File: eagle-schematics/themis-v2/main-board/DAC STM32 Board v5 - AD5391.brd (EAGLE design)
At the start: 161.3 x 134.6 mm, 229 parts, among them IC1 MCP23017SO, U1 ANALOG_DEVICES_AD5391BSTZ-3AN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

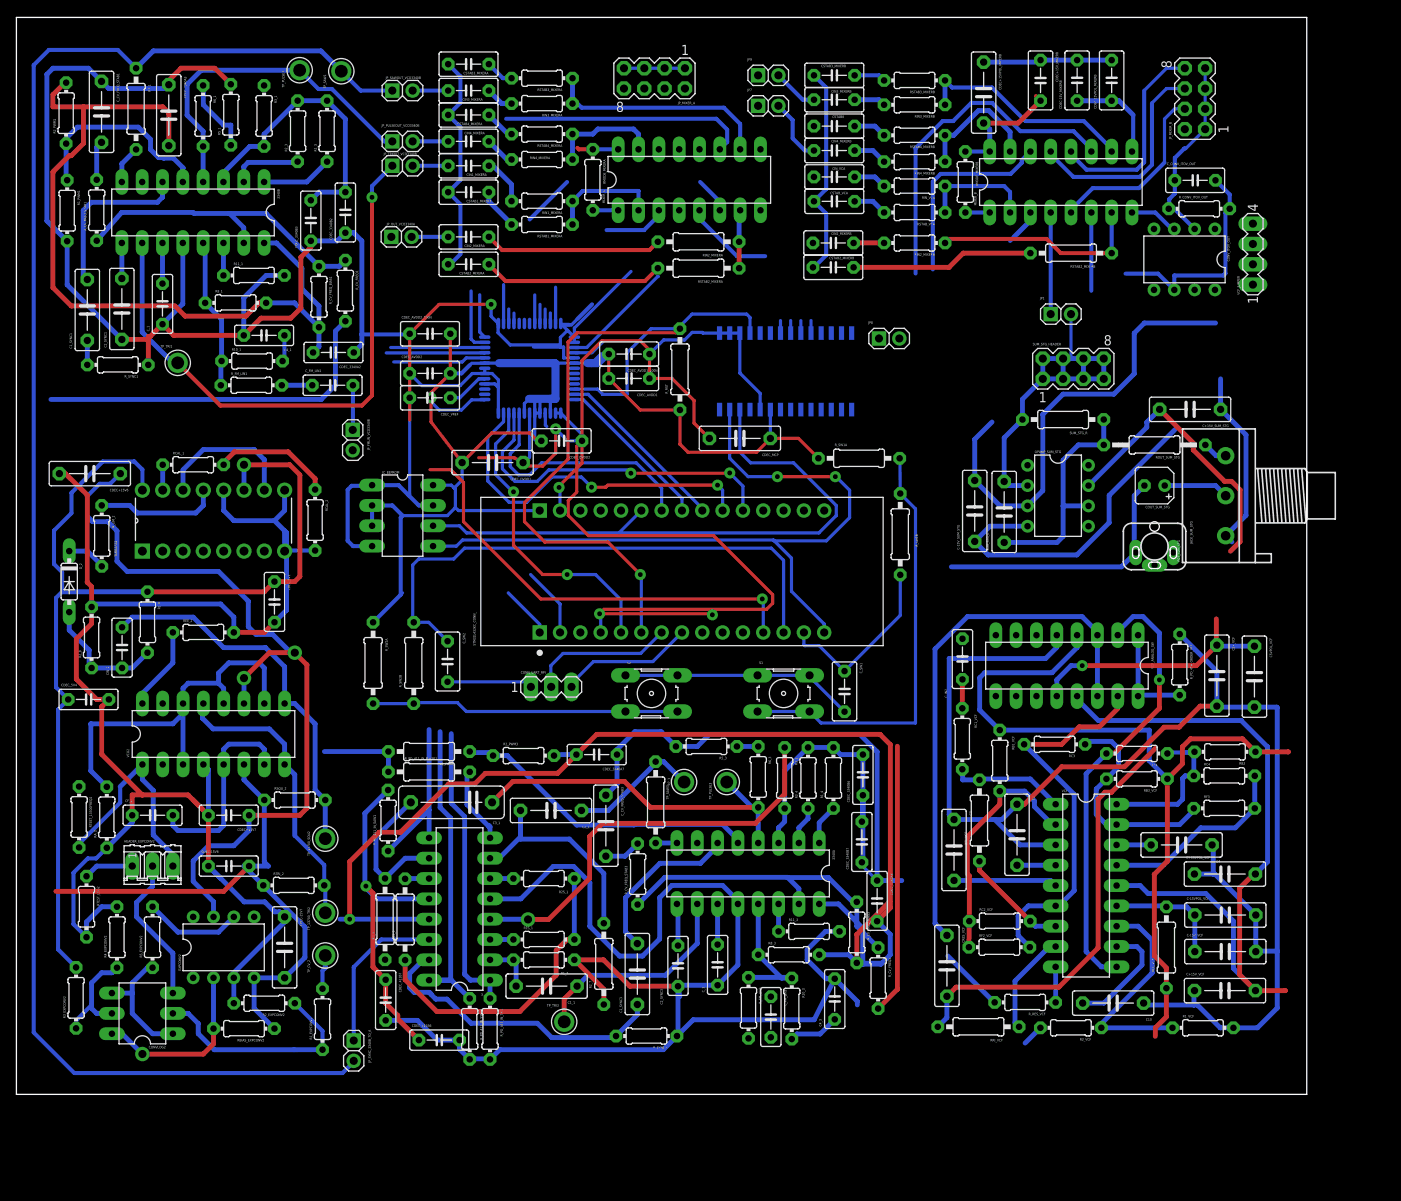
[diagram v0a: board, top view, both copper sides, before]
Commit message: bug fix
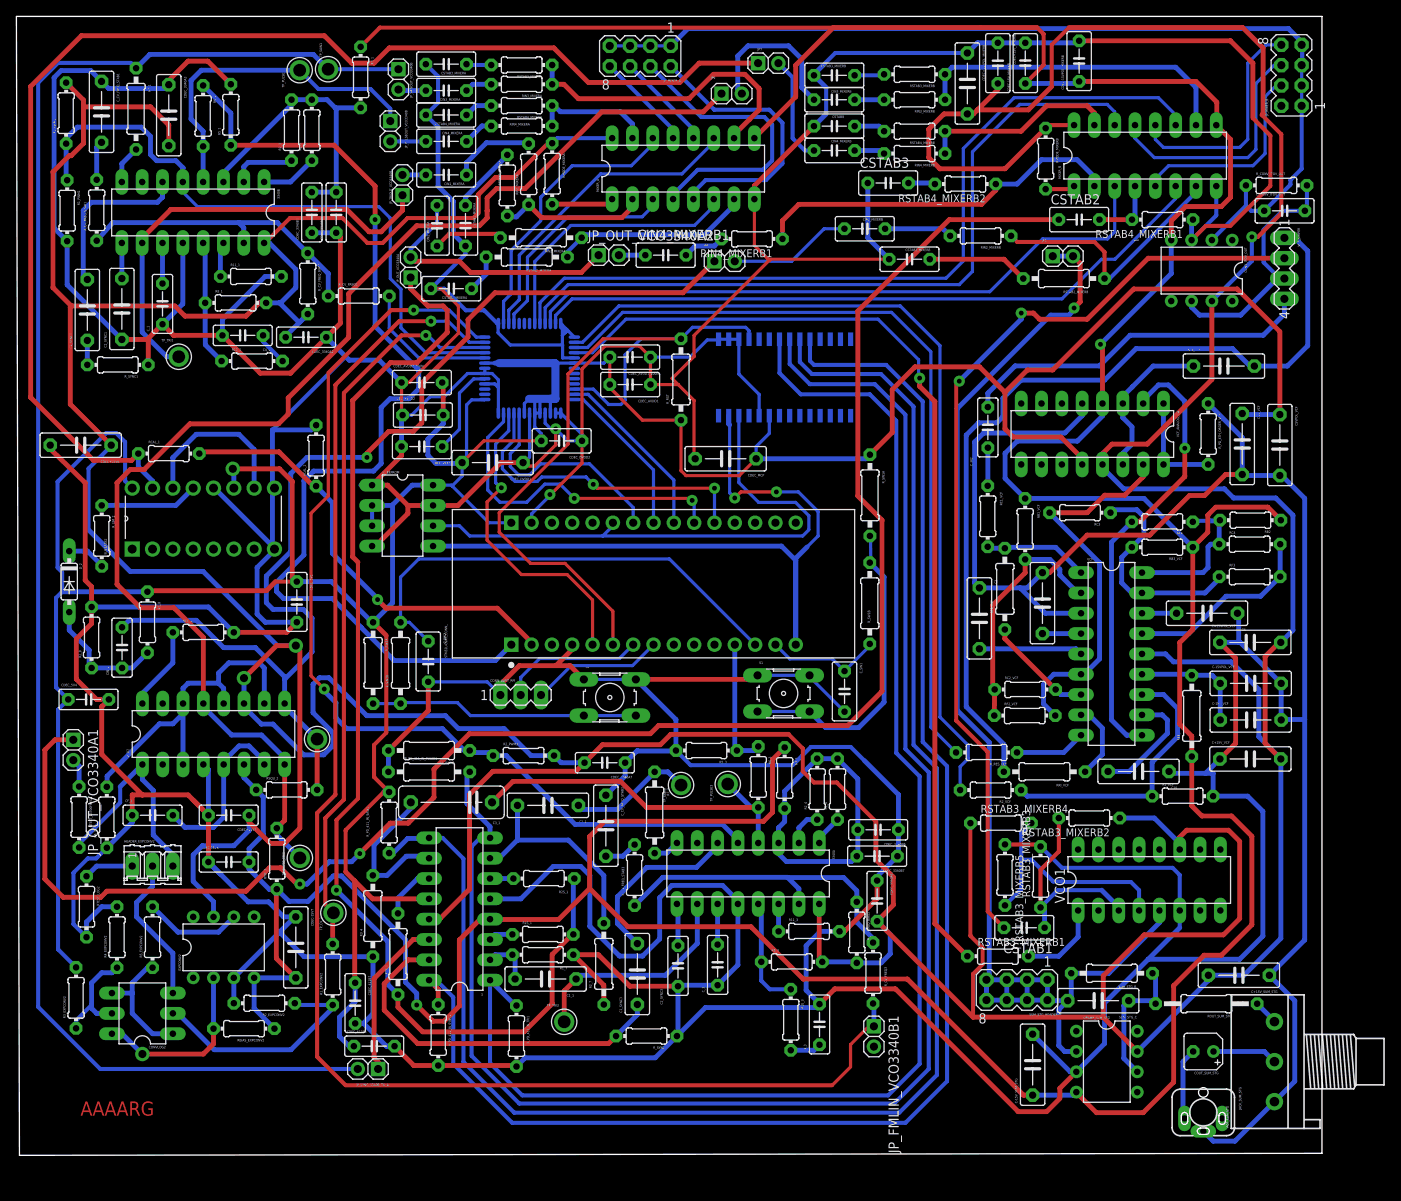
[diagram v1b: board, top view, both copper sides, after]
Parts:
- removed CIN_VCA: 470n, rcl:C050-030X075
- removed CSTAB_VCA: 560p, rcl:C050-030X075
- removed C_FM_LIN1, C_FM_LIN3: 100n, rcl:C050-025X075
- removed JP_FMLIN_VCO3340B: JUMPER, 6P1_EVB:HDR2X1
- removed RIN_VCA: 27k, rcl:0204/7
- removed RSTAB_VCA: 470, rcl:0204/7
- removed R_FM_LIN1, R_FM_LIN3: 1M, rcl:0204/7
- added CIN4_MIXERB1: 470n, rcl:C050-030X075
- added CSTAB1: 10u, rcl:C050-030X075
- added CSTAB2, CSTAB3: 560p, rcl:C050-030X075
- added JP_FMLIN_VCO3340B1, JP_OUT_VCO3340A1, JP_OUT_VCO3340A2: JUMPER, 6P1_EVB:HDR2X1
- added RIN4_MIXERB1: 27k, rcl:0204/7
- added RSTAB3_MIXERB1: 51k, rcl:0204/7
- added RSTAB3_MIXERB2, RSTAB3_MIXERB3, RSTAB3_MIXERB4, RSTAB3_MIXERB5: 10k, rcl:0204/7
- added RSTAB4_MIXERB1, RSTAB4_MIXERB2: 470, rcl:0204/7
- added VCO1: LM13700N, ota:DIL16
- moved CRES_VCF 82.6 mm to (150.9, 91.0), turned to 0 degrees
- moved SUM_STG_HEADER 78.0 mm to (125.1, 13.1), turned to 180 degrees
- moved COUT_SUM_STG 71.0 mm to (148.4, 5.36)
- moved JACK_SUM_STG 71.0 mm to (148.4, -2.26)
- moved C+15V_SUM_STG 71.0 mm to (152.8, 14.9)
- moved OPAMP_SUM_STG 71.0 mm to (136.3, 4.09)
- moved POT_SUM_STG 71.0 mm to (157.3, 4.09)
- moved ROUT_SUM_STG 70.1 mm to (148.7, 11.3)
- moved C-15V_SUM_STG 69.6 mm to (127.0, 3.71)
- moved SUM_STG_R 69.5 mm to (136.9, 15.1)
- moved SUM_STG_C 62.2 mm to (135.2, 11.7), turned to 180 degrees
- moved RRI_VCF 32.9 mm to (128.5, 40.3)
- moved R_RES_VCF 31.6 mm to (121.3, 42.7)
- moved R2_VCF 31.4 mm to (121.8, 38.0)
- moved C-15V_VCF 29.1 mm to (154.3, 46.8)
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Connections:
- removed net 2164_IN1_MIXB: MIXER_B.2, RIN_VCA.1, RSTAB_VCA.1
- removed net 2164_OUT1_MIXA: JP_MIXER_A.2, MIXER_A.4
- removed net CSTAB3_MIXERB: CSTAB8.1
- removed net N$21: CSTAB_VCA.2, RSTAB_VCA.2
- removed net N$62: CIN_VCA.2, RIN_VCA.2
- removed net N$84: C_FM_LIN1.1, R_FM_LIN1.2
- removed net N$92: C_FM_LIN3.1, R_FM_LIN3.2
- removed net N$93: C_FM_LIN3.2
- removed net NOISE_GENE: U1.30
- removed net OUT_VCA: JP1.1, MIXER_B.4
- removed net VCO3340B_FMLIN: C_FM_LIN1.2, JP_FMLIN_VCO3340B.1
- new net 2164_IN4_MIXB1: MIXER_B.2, RIN4_MIXERB1.1, RSTAB4_MIXERB2.1
- new net CV_VCA: RSTAB3_MIXERB1.1, U1.30
- new net IN4_MIXERB1: CIN4_MIXERB1.1, JP_OUT_VCO3340A2.2
- new net N$10: CSTAB3.2, RSTAB4_MIXERB2.2
- new net N$11: CIN4_MIXERB1.2, RIN4_MIXERB1.2
- new net N$12: RSTAB3_MIXERB4.2, RSTAB3_MIXERB5.2, VCO1.4
- new net N$17: RSTAB3_MIXERB1.2, VCO1.1
- new net N$2: JP_FMLIN_VCO3340B1.2
- new net N$4: JP_MIXER_A.4, MIXER_A.4
- new net N$8: CSTAB2.2, MIXER_B.4, RSTAB4_MIXERB1.2
- new net N$9: CSTAB1.1, RSTAB3_MIXERB2.2, RSTAB3_MIXERB3.1, VCO1.3
- net +15V: now also RSTAB3_MIXERB2.1, RSTAB3_MIXERB4.1, VCO1.11
- net 2164_OUT2_MIXA: now also JP_MIXER_A.2; no longer JP_MIXER_A.4
- net 2164_OUT3_MIXA: now also JP_MIXER_A.6; no longer JP_MIXER_A.8
- net 2164_OUT4_MIXA: now also JP_MIXER_A.8; no longer JP_MIXER_A.6
- net 411_IN_PULSE: now also IC1.22; no longer IC1.21
- net 411_IN_SAW: now also IC1.23; no longer IC1.24
- net 411_IN_SYNC: now also IC1.24; no longer IC1.23
- net 411_IN_TRI: now also IC1.21; no longer IC1.22
- net AGND: now also CSTAB3.1, CSTAB8.1, RSTAB3_MIXERB3.2, RSTAB3_MIXERB5.1, RSTAB4_MIXERB1.1, VCO1.6; no longer CSTAB_VCA.1
- net CV_FREQ_3340A: now also JP_FMLIN_VCO3340B1.1
- net GAIN3_A: now also U1.16; no longer U1.15
- net GAIN4_A: now also U1.15; no longer U1.16
- net IN2_MIXERA: now also JP_OUT_VCO3340A2.1
- net INPUT_CURRENT_SUM_STG: now also JP1.1, VCO1.5
- net INPUT_FM_3340: now also JP_OUT_VCO3340A1.2
- net IN_VCA: now also CSTAB1.2; no longer CIN_VCA.1
- net LINEAR_CTRL_VCOA: no longer R_FM_LIN3.1
- net LINEAR_CTRL_VCOB: no longer R_FM_LIN1.1
- net N$1: now also CSTAB2.1, JP_OUT_VCO3340A1.1; no longer JP_FMLIN_VCO3340B.2
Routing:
- net +15V: track 506.5 -> 843.6 mm
- net -15V: track 280.1 -> 577.0 mm, vias 1 -> 2
- net AGND: track 1271.4 -> 1515.6 mm, vias 5 -> 2
- net N$1: track 0.00 -> 218.9 mm, vias 0 -> 2
- net 411_IN_PULSE: track 11.4 -> 203.1 mm
- net 411_IN_SAW: track 22.4 -> 204.4 mm
- net VCO13700_SUBBASS: track 3.17 -> 159.6 mm
- net 411_IN_SYNC: track 41.8 -> 187.8 mm
- net CV_FREQ_3340A: track 41.7 -> 186.6 mm, vias 0 -> 1
- net 411_IN_TRI: track 38.1 -> 174.9 mm
- net VCO13700_TRI: track 36.7 -> 163.4 mm
- net CV_VCA: track 0.00 -> 123.9 mm, vias 0 -> 1
- net IN_VCA: track 0.00 -> 119.3 mm, vias 0 -> 2
- net CALIB_3340B: track 16.0 -> 128.9 mm, vias 0 -> 1
- net INPUT_CURRENT_SUM_STG: track 49.6 -> 160.7 mm, vias 0 -> 1
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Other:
- board size 161.3 x 134.6 mm -> 163.2 x 142.4 mm
- board text added: "AAAARG"
